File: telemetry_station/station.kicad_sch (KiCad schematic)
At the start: 32 parts, among them J9 USB_C_Receptacle_USB2.0_16P, SW2 SW_Push, U11 SX1280IMLTRT, U14 STM32G0B1CBTx, U15 TLV75533PDBV, U16 WE-TVS-82400102, Y2 52Mhz, Y5 8Mhz

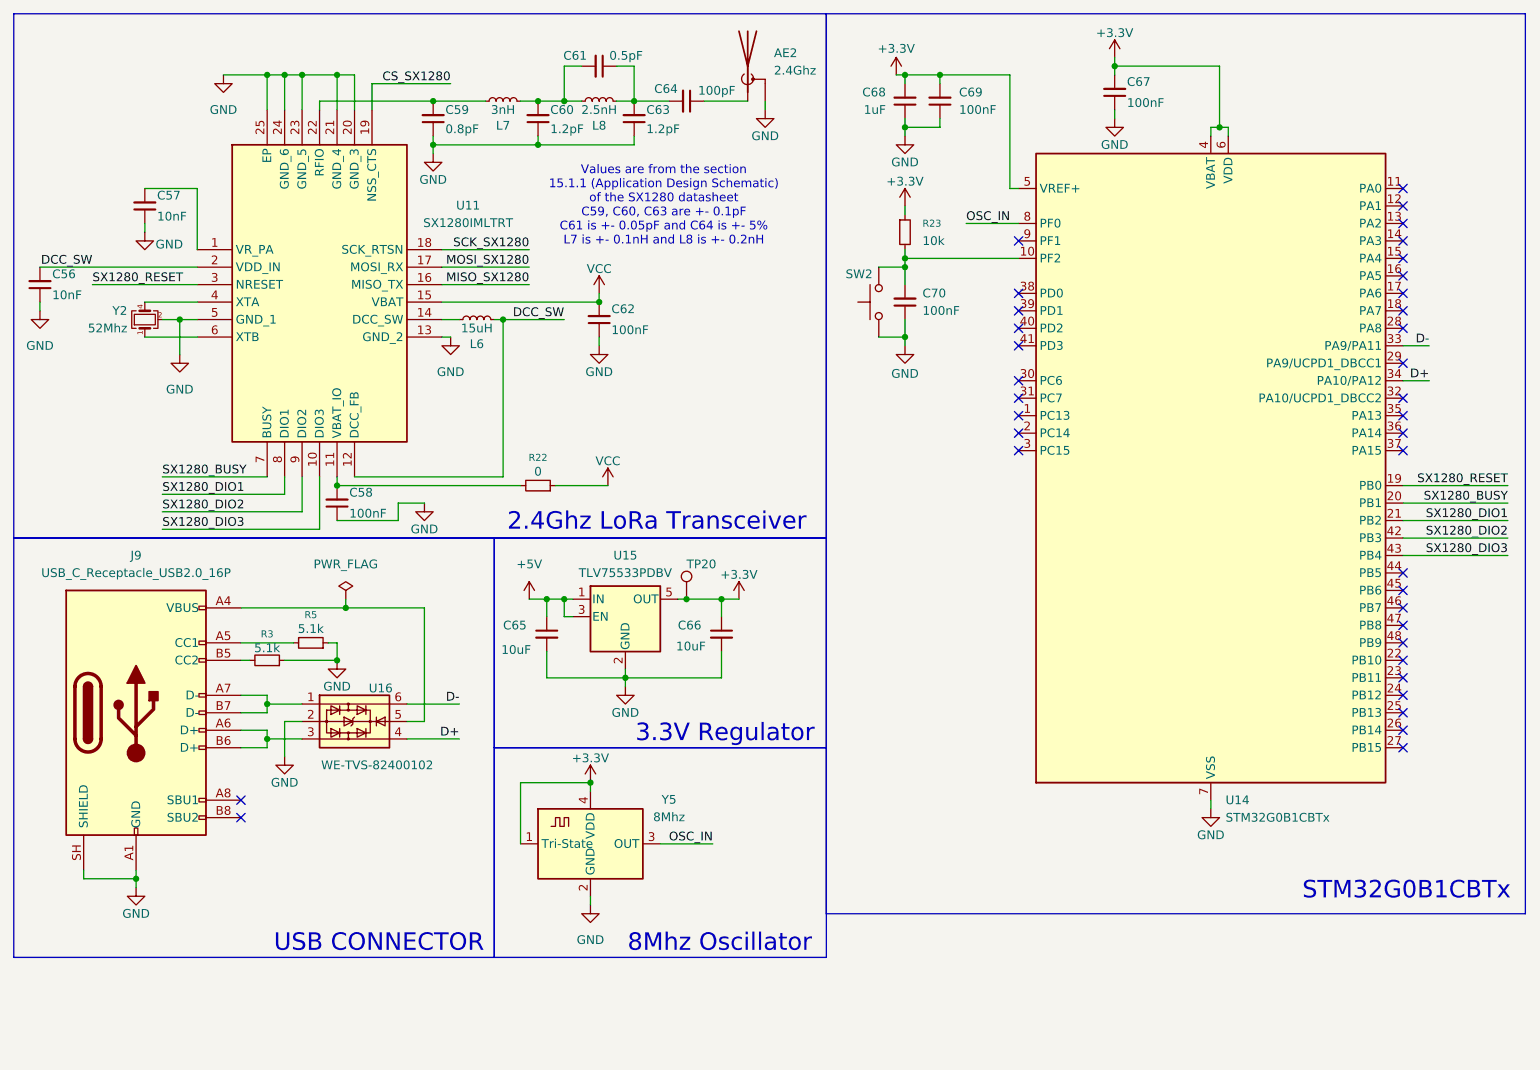
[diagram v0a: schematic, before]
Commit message: Arduino SHIELD
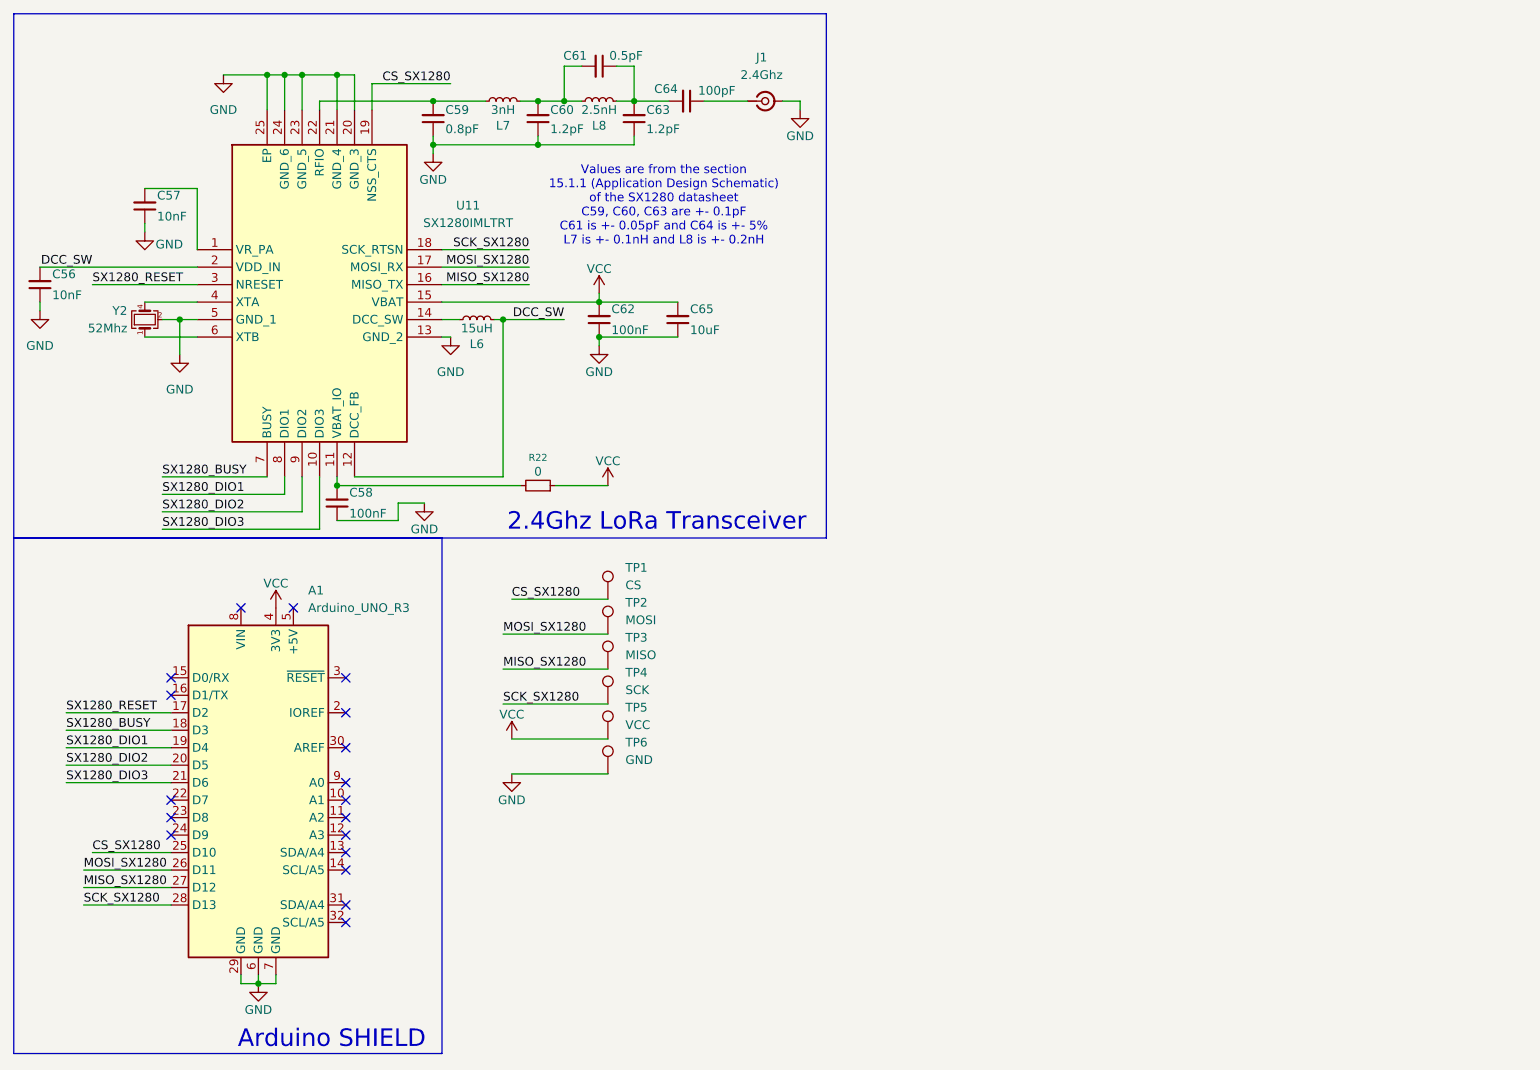
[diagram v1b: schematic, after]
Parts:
- removed AE2: 2.4Ghz, symbol Device:Antenna_Shield
- removed C66: 10uF, Capacitor_SMD:C_1206_3216Metric, symbol Device:C_Small
- removed C67, C69, C70: 100nF, Capacitor_SMD:C_1206_3216Metric, symbol Device:C_Small
- removed C68: 1uF, Capacitor_SMD:C_1206_3216Metric, symbol Device:C_Small
- removed J9: USB_C_Receptacle_USB2.0_16P, Connector_USB:USB_C_Receptacle_GCT_USB4105-xx-A_16P_TopMnt_Horizontal, symbol Connector:USB_C_Receptacle_USB2.0_16P
- removed R23: 10k, Resistor_SMD:R_1206_3216Metric, symbol Device:R_Small
- removed R3, R5: 5.1k, Resistor_SMD:R_1206_3216Metric, symbol Device:R_Small
- removed SW2: SW_Push, Button_Switch_SMD:Nidec_Copal_CAS-120A, symbol Switch:SW_Push
- removed TP20: VCC, TestPoint:TestPoint_THTPad_1.0x1.0mm_Drill0.5mm, symbol Connector:TestPoint
- removed U14: STM32G0B1CBTx, Package_QFP:LQFP-48_7x7mm_P0.5mm, symbol MCU_ST_STM32G0:STM32G0B1CBTx
- removed U15: TLV75533PDBV, Package_TO_SOT_SMD:SOT-23-5, symbol Regulator_Linear:TLV75533PDBV
- removed U16: WE-TVS-82400102, Package_TO_SOT_SMD:SOT-23-6, symbol Power_Protection:WE-TVS-82400102
- removed Y5: 8Mhz, Oscillator:Oscillator_SMD_Abracon_ASCO-4Pin_1.6x1.2mm, symbol Oscillator:ASCO
- added A1: Arduino_UNO_R3, Module:Arduino_UNO_R3, symbol MCU_Module:Arduino_UNO_R3
- added J1: 2.4Ghz, Connector_Coaxial:SMA_Amphenol_132134_Vertical, symbol Connector:Conn_Coaxial_Small
- added TP1: CS, TestPoint:TestPoint_Pad_D1.0mm, symbol Connector:TestPoint
- added TP2: MOSI, TestPoint:TestPoint_Pad_D1.0mm, symbol Connector:TestPoint
- added TP3: MISO, TestPoint:TestPoint_Pad_D1.0mm, symbol Connector:TestPoint
- added TP4: SCK, TestPoint:TestPoint_Pad_D1.0mm, symbol Connector:TestPoint
- added TP5: VCC, TestPoint:TestPoint_Pad_D1.0mm, symbol Connector:TestPoint
- added TP6: GND, TestPoint:TestPoint_Pad_D1.0mm, symbol Connector:TestPoint
- C59, C60, C61, C63, C64: footprint Capacitor_SMD:C_1206_3216Metric -> Capacitor_SMD:C_0402_1005Metric
- L6: footprint (none) -> Inductor_SMD:L_0603_1608Metric
- L7, L8: footprint (none) -> Inductor_SMD:L_0402_1005Metric
- Y2: footprint QFN50P400X400X100-25N-D -> Crystal:Crystal_SMD_2016-4Pin_2.0x1.6mm
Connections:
- net +5V is gone; now on net GND: C65.1
- net CS_SX1280: now also A1.25 (D10), TP1.1
- net GND: now also A1.29 (GND), A1.6 (GND), A1.7 (GND), J1.2 (Ext), TP6.1; no longer C65.2
- net MISO_SX1280: now also A1.27 (D12), TP3.1
- net MOSI_SX1280: now also A1.26 (D11), TP2.1
- net SCK_SX1280: now also A1.28 (D13), TP4.1
- net SX1280_BUSY: now also A1.18 (D3)
- net SX1280_DIO1: now also A1.19 (D4)
- net SX1280_DIO2: now also A1.20 (D5)
- net SX1280_DIO3: now also A1.21 (D6)
- net SX1280_RESET: now also A1.17 (D2)
- net VCC: now also C65.2, A1.4 (3V3), TP5.1
- net at C64.1: now also J1.1 (In)
- no-connect marks 37 -> 18
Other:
- note added: "Arduino SHIELD"
- note removed: "3.3V Regulator"
- note removed: "8Mhz Oscillator"
- note removed: "STM32G0B1CBTx"
- note removed: "USB CONNECTOR"
